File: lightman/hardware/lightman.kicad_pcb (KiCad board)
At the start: 2 copper layers, 139 x 80 mm, 39 parts, among them J1 DE15_Socket_HighDensity_Mount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, J2 Mini-DIN-6, J4 DE9_Pins, J5 Barrel_Jack_Switch, SW23 POWER, U1 MAX3232, U2 L7805, U3 MAX3232

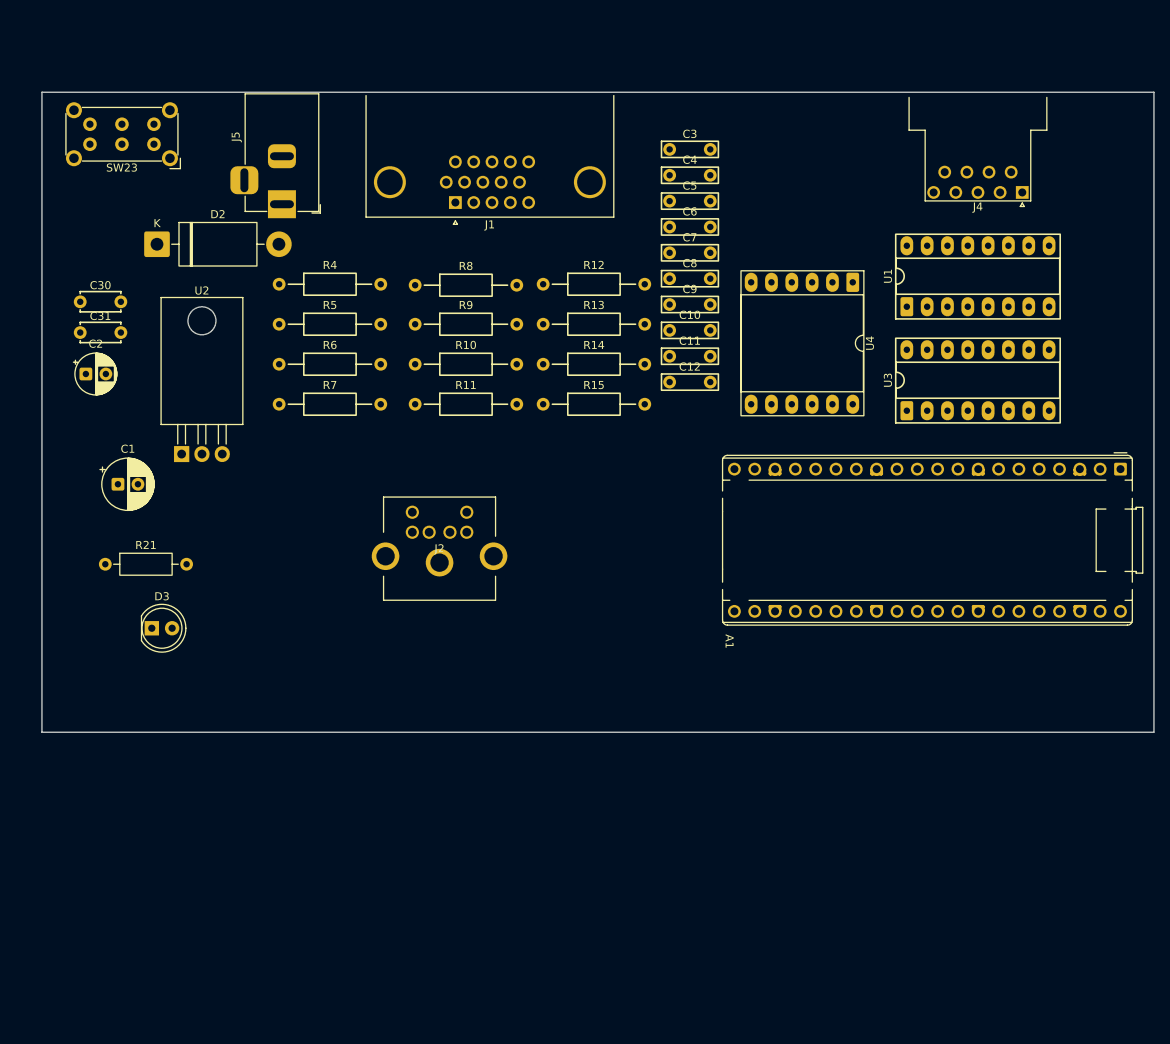
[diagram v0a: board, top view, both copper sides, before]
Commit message: lightman pcb
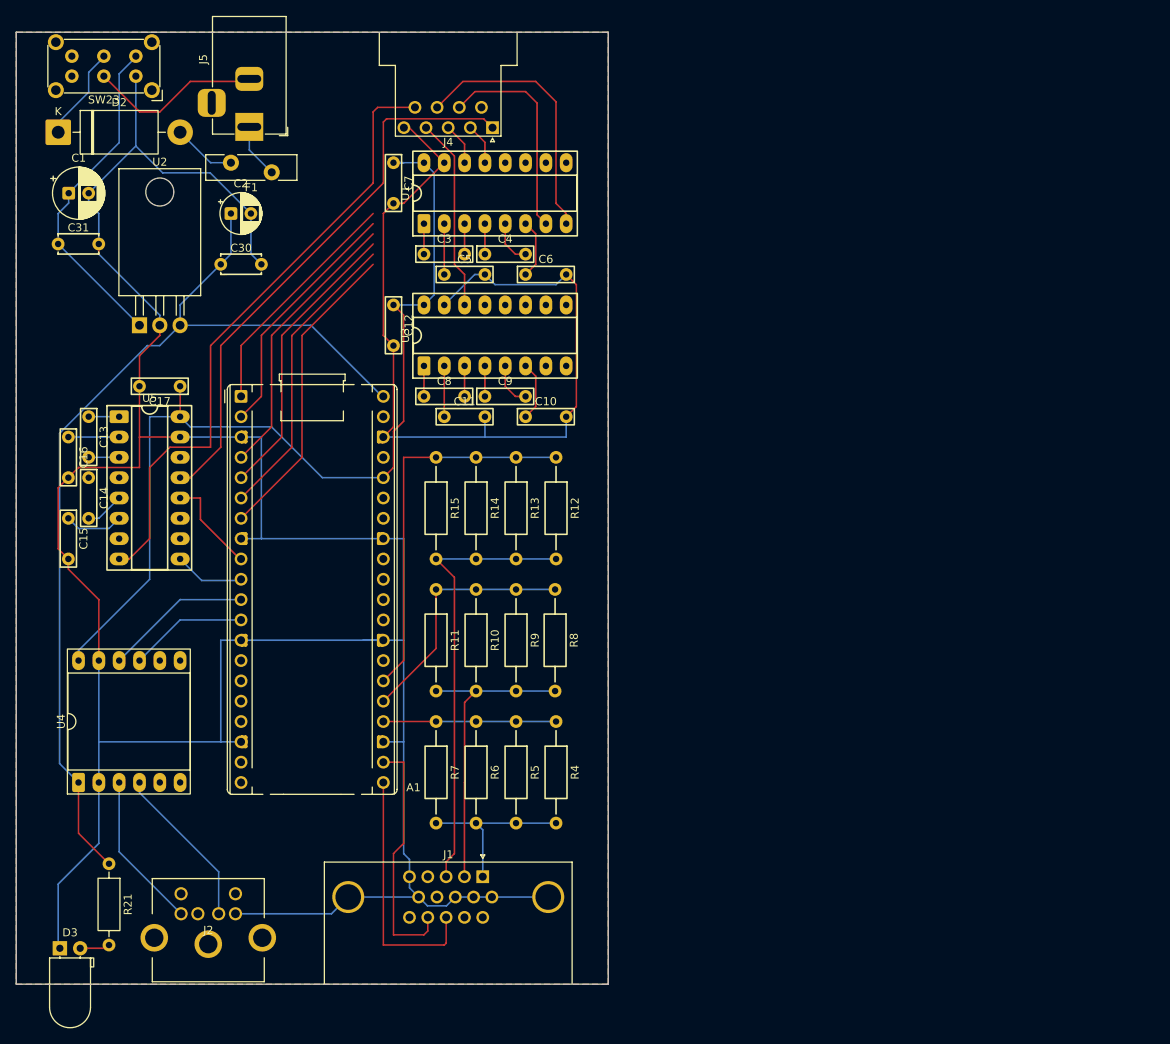
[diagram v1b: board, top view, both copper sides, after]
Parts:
- added C13: 100n, IMNOTWOPR:C_Rect_P200mil, F.Cu at (71.8, 93.1)
- added C14: 100n, IMNOTWOPR:C_Rect_P200mil, F.Cu at (71.8, 100.7)
- added C15: 100n, IMNOTWOPR:C_Rect_P200mil, F.Cu at (69.3, 105.8)
- added C16: 100n, IMNOTWOPR:C_Rect_P200mil, F.Cu at (69.3, 95.6)
- added C17: 100n, IMNOTWOPR:C_Rect_P200mil, F.Cu at (80.7, 86.7)
- added F1: Polyfuse, Fuse:Fuse_Bourns_MF-RG700, F.Cu at (94.7, 60.0)
- added U5: MAX3232, IMNOTWOPR:DIP-16N, F.Cu at (79.5, 99.4)
- D3: footprint LED_THT:LED_D5.0mm -> LED_THT:LED_D5.0mm_Horizontal_O1.27mm_Z3.0mm
- R21: value 470 -> 1k
- U4: value ~ -> LEVEL SHIFTER
- moved A1 110.3 mm to (90.9, 88.0), turned to 0 degrees
- moved U4 96.5 mm to (76.9, 128.7), turned to 90 degrees
- moved J1 84.3 mm to (121.1, 148.1), turned to 0 degrees
- moved R4 67.2 mm to (130.3, 135.0), turned to -90 degrees
- moved J4 66.7 mm to (122.3, 54.4)
- moved U1 61.2 mm to (122.6, 62.6)
- moved R5 60.6 mm to (125.3, 135.0), turned to -90 degrees
- moved U3 60.6 mm to (122.6, 80.4)
- moved J2 55.8 mm to (88.1, 152.7)
- moved R6 54.2 mm to (120.3, 135.0), turned to -90 degrees
- moved R7 47.9 mm to (115.3, 135.0), turned to -90 degrees
- moved R8 45.8 mm to (130.1, 118.5), turned to -90 degrees
- moved R21 42.8 mm to (74.4, 151.5), turned to -90 degrees
- moved D3 41.6 mm to (68.2, 157.0)
- moved R9 40.0 mm to (125.3, 118.5), turned to -90 degrees
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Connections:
- A1 pad 10: /KEY_DATA_LO -> /PICO_RI
- A1 pad 11: unconnected-(A1-GPIO8-Pad11) -> /KEY_CLOCK_LO
- A1 pad 12: unconnected-(A1-GPIO9-Pad12) -> /KEY_DATA_LO
- A1 pad 9: /KEY_CLOCK_LO -> /PICO_DCD
- J4 pad 9: unconnected-(J4-Pad9) -> /RI
- J5 pad 1: Net-(D2-A) -> Net-(F1-Pad1)
- R21 pad 1: +9V -> +5V
- U3 pad 12: unconnected-(U3-R1OUT-Pad12) -> /PICO_DSR
- U3 pad 13: /DCD -> /DSR
- U3 pad 7: /RTR -> unconnected-(U3-T2OUT-Pad7)
- U3 pad 8: /DSR -> unconnected-(U3-R2IN-Pad8)
- U3 pad 9: /PICO_DSR -> unconnected-(U3-R2OUT-Pad9)
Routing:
- net GND: track 0.00 -> 457.9 mm
- net +5V: track 0.00 -> 122.8 mm
- net +3V3: track 0.00 -> 121.2 mm
- net /RI: track 0.00 -> 78.2 mm
- net /DCD: track 0.00 -> 70.0 mm
- net /BLUE: track 0.00 -> 56.1 mm
- net Net-(A1-GPIO20): track 0.00 -> 48.0 mm
- net +9V: track 0.00 -> 41.9 mm
- net /GREEN: track 0.00 -> 38.7 mm
- net /PICO_DSR: track 0.00 -> 38.6 mm
- net /PICO_DTR: track 0.00 -> 37.3 mm
- net /PICO_RTS: track 0.00 -> 36.0 mm
- net /PICO_CTS: track 0.00 -> 34.8 mm
- net /CTS: track 0.00 -> 33.0 mm
- net Net-(A1-GPIO19): track 0.00 -> 31.6 mm
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- added copper zone on B.Cu, net GND
- added copper zone on F.Cu, net GND
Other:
- board size 139 x 80 mm -> 74 x 119 mm
- board text added: "${COMPANY}"

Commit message: lightman pcb
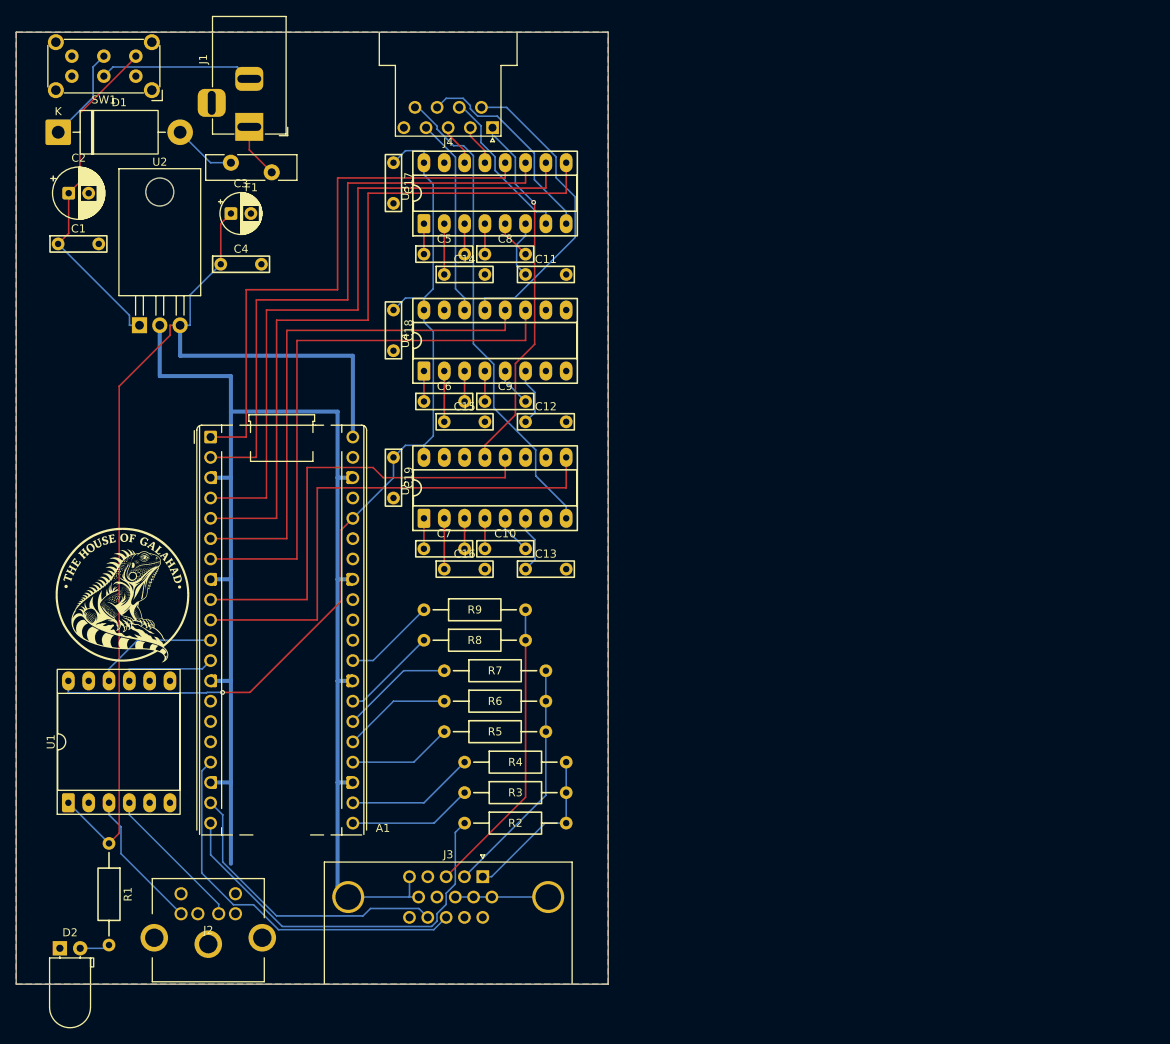
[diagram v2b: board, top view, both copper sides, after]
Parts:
- removed R12, R13, R14, R15: 1k, IMNOTWOPR:R_Axial_DIN0207_P400mil
- C1: renamed from C31; footprint Desval27:C_Disc_D5.0mm_W2.5mm_P200mil -> IMNOTWOPR:C_Rect_P200mil
- C4: renamed from C30; footprint Desval27:C_Disc_D5.0mm_W2.5mm_P200mil -> IMNOTWOPR:C_Rect_P200mil
- R1: renamed from R21; footprint Desval27:R_Axial_DIN0207_400mil -> IMNOTWOPR:R_Axial_DIN0207_P400mil
- R2: renamed from R4; value 1k -> 470R
- R4: renamed from R6; value 1k -> 2k2
- R5: renamed from R7; value 1k -> 470R
- R7: renamed from R9; value 1k -> 2k2
- R8: renamed from R10; value 1k -> 390R
- moved C13 59.8 mm to (129.0, 109.6), turned to 0 degrees
- moved C10 52.5 mm to (123.9, 107.1), turned to 0 degrees
- moved C16 51.5 mm to (118.8, 109.6), turned to 0 degrees
- moved C7 46.6 mm to (116.3, 107.1), turned to 0 degrees
- moved U5 43.2 mm to (122.6, 99.5), turned to 90 degrees
- moved C19 31.4 mm to (109.9, 98.2), turned to -90 degrees
- moved R6 10.7 mm to (122.6, 126.1), turned to 0 degrees
- moved R5 8.96 mm to (122.6, 129.9), turned to 0 degrees
- moved R2 8.13 mm to (125.2, 141.4), turned to 0 degrees
- moved A1 6.35 mm to (87.1, 93.1)
- moved R9 6.16 mm to (120.1, 114.7), turned to 0 degrees
- moved R4 5.08 mm to (125.2, 133.7), turned to 0 degrees
- moved R7 4.62 mm to (122.6, 122.3), turned to 0 degrees
- moved U1 2.84 mm to (75.7, 131.2)
- moved R3 2.54 mm to (125.2, 137.6), turned to 0 degrees
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- renumbered C14 to C10, C6 to C11, C10 to C12, C15 to C13, C5 to C14, C11 to C15, C7 to C17, C12 to C18, C17 to C19, C1 to C2, C2 to C3, C3 to C5, C8 to C6, C13 to C7, C4 to C8, D2 to D1, D3 to D2, J5 to J1, J1 to J3, R5 to R3, R8 to R6, R11 to R9, SW23 to SW1, U4 to U1, U1 to U3, U3 to U4
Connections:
- A1 pad 1: /PICO_TXD -> /PICO_RXD
- A1 pad 17: unconnected-(A1-GPIO13-Pad17) -> /HSYNC
- A1 pad 19: unconnected-(A1-GPIO14-Pad19) -> /VSYNC
- A1 pad 2: /PICO_RXD -> /PICO_TXD
- A1 pad 20: unconnected-(A1-GPIO15-Pad20) -> /R0
- A1 pad 21: /HSYNC -> /R1
- A1 pad 22: /VSYNC -> /R2
- A1 pad 24: Net-(A1-GPIO18) -> /G0
- A1 pad 25: Net-(A1-GPIO19) -> /G1
- A1 pad 26: Net-(A1-GPIO20) -> /G2
- A1 pad 27: unconnected-(A1-GPIO21-Pad27) -> /B0
- A1 pad 29: unconnected-(A1-GPIO22-Pad29) -> /B1
- A1 pad 4: /PICO_CTS -> /PICO_RTS
- A1 pad 5: /PICO_RTS -> /PICO_CTS
- A1 pad 6: /PICO_DTR -> /PICO_DSR
- A1 pad 7: /PICO_DSR -> /PICO_DTR
- R2 pad 1: Net-(A1-GPIO18) -> /R0
- R3 pad 1: Net-(A1-GPIO18) -> /R1
- R4 pad 1: Net-(A1-GPIO18) -> /R2
- R5 pad 1: Net-(A1-GPIO18) -> /G0
- R5 pad 2: /RED -> /GREEN
- R6 pad 1: Net-(A1-GPIO19) -> /G1
- R7 pad 1: Net-(A1-GPIO19) -> /G2
- R8 pad 1: Net-(A1-GPIO19) -> /B0
- R8 pad 2: /GREEN -> /BLUE
- R9 pad 1: Net-(A1-GPIO19) -> /B1
- R9 pad 2: /GREEN -> /BLUE
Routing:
- net GND: track 457.9 -> 191.5 mm
- net /PICO_RI: track 8.74 -> 64.8 mm
- net /PICO_CTS: track 34.8 -> 88.9 mm
- net /R0: track 0.00 -> 49.9 mm
- net Net-(A1-GPIO20): track 48.0 -> 0.00 mm
- net /PICO_RTS: track 36.0 -> 83.8 mm
- net /PICO_TXD: track 29.7 -> 76.2 mm
- net /PICO_DCD: track 12.4 -> 56.4 mm
- net /PICO_RXD: track 31.0 -> 71.1 mm
- net /DSR: track 0.00 -> 38.9 mm
- net /PICO_DTR: track 37.3 -> 70.5 mm
- net Net-(A1-GPIO19): track 31.6 -> 0.00 mm
- net /PICO_DSR: track 38.6 -> 65.4 mm
- net /DCD: track 70.0 -> 46.1 mm, vias 0 -> 1
- net Net-(A1-GPIO18): track 21.6 -> 0.00 mm
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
